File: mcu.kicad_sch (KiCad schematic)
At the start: 15 parts, among them J2 Conn_01x05_Pin, J3 Conn_01x10_Pin, J5 Conn_01x04, J6 Conn_01x04, SW1 SWT0010-015016SSA, SW2 SWT0010-015016SSA, U301 ESP32-C6-MINI-1

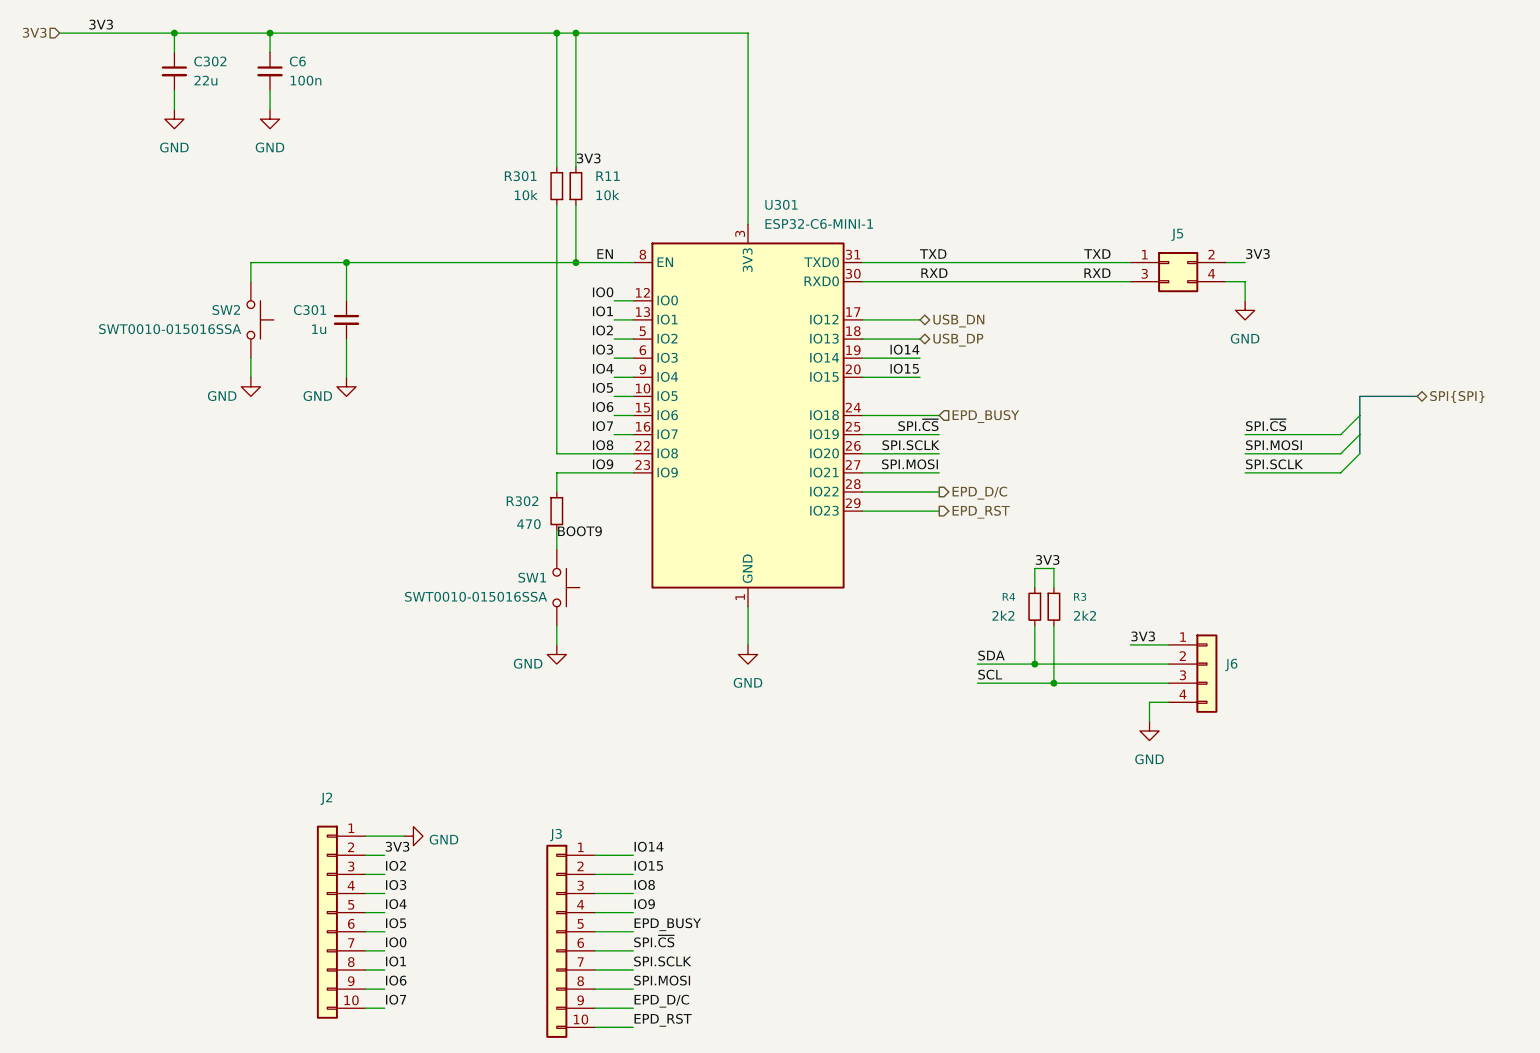
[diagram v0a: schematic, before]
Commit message: WIP
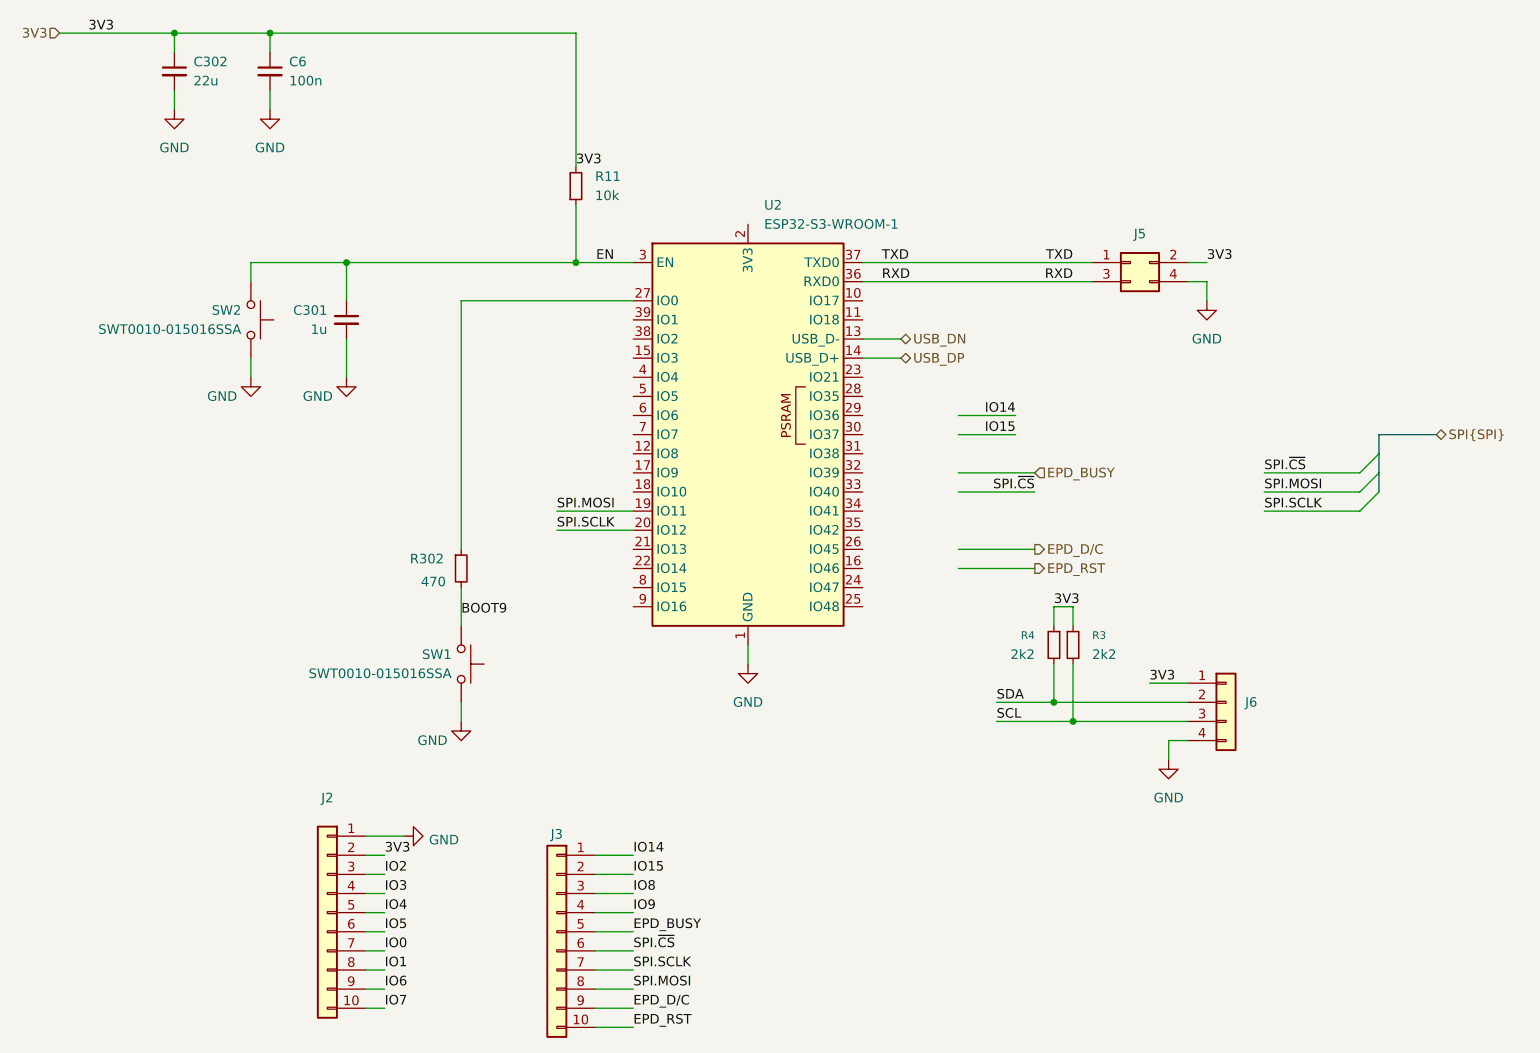
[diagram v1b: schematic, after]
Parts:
- removed R301: 10k, Resistor_SMD:R_0805_2012Metric, symbol Device:R_Small
- removed U301: ESP32-C6-MINI-1, RF_Module:ESP32-C6-MINI-1, symbol RF_Module:ESP32-C6-MINI-1
- added U2: ESP32-S3-WROOM-1, RF_Module:ESP32-S3-WROOM-1, symbol RF_Module:ESP32-S3-WROOM-1
- J6: footprint (none) -> Connector_PinHeader_2.54mm:PinHeader_1x04_P2.54mm_Vertical
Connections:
- net EN: now also U2.3 (EN)
- net GND: now also U2.1 (GND), U2.40 (GND), U2.41 (GND)
- net IO9: no longer R302.1
- net RXD: now also U2.36 (RXD0)
- net SPI.MOSI: now also U2.19 (IO11)
- net SPI.SCLK: now also U2.20 (IO12)
- net TXD: now also U2.37 (TXD0)
- net USB_DN: now also U2.13 (USB_D-)
- net USB_DP: now also U2.14 (USB_D+)
- new net: R302.1, U2.27 (IO0)
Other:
- moved on the sheet: J5, J6, R3, R302, R4, SW1
